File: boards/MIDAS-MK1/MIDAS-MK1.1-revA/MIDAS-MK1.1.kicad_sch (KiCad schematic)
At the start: 105 parts, among them J101 Left, J102 Right, J106 USB4105-GF-A, J107 DM3BT-DSF-PEJS, J108 Conn_01x02, J110 2157601003, J111 2157601003, SW101 SW_Push, SW102 SW_Push, U101 TCAL9539-Q1, U102 TCAL9539-Q1, U103 TCAL9539-Q1, U104 ESP32-S3-WROOM-1U, U105 MCP2518FDT-xSL, U106 MTFCxxxx, U107 TCAN337G, U108 ADS7138-Q1, U109 ECMF02-2AMX6, Y101 40MHz

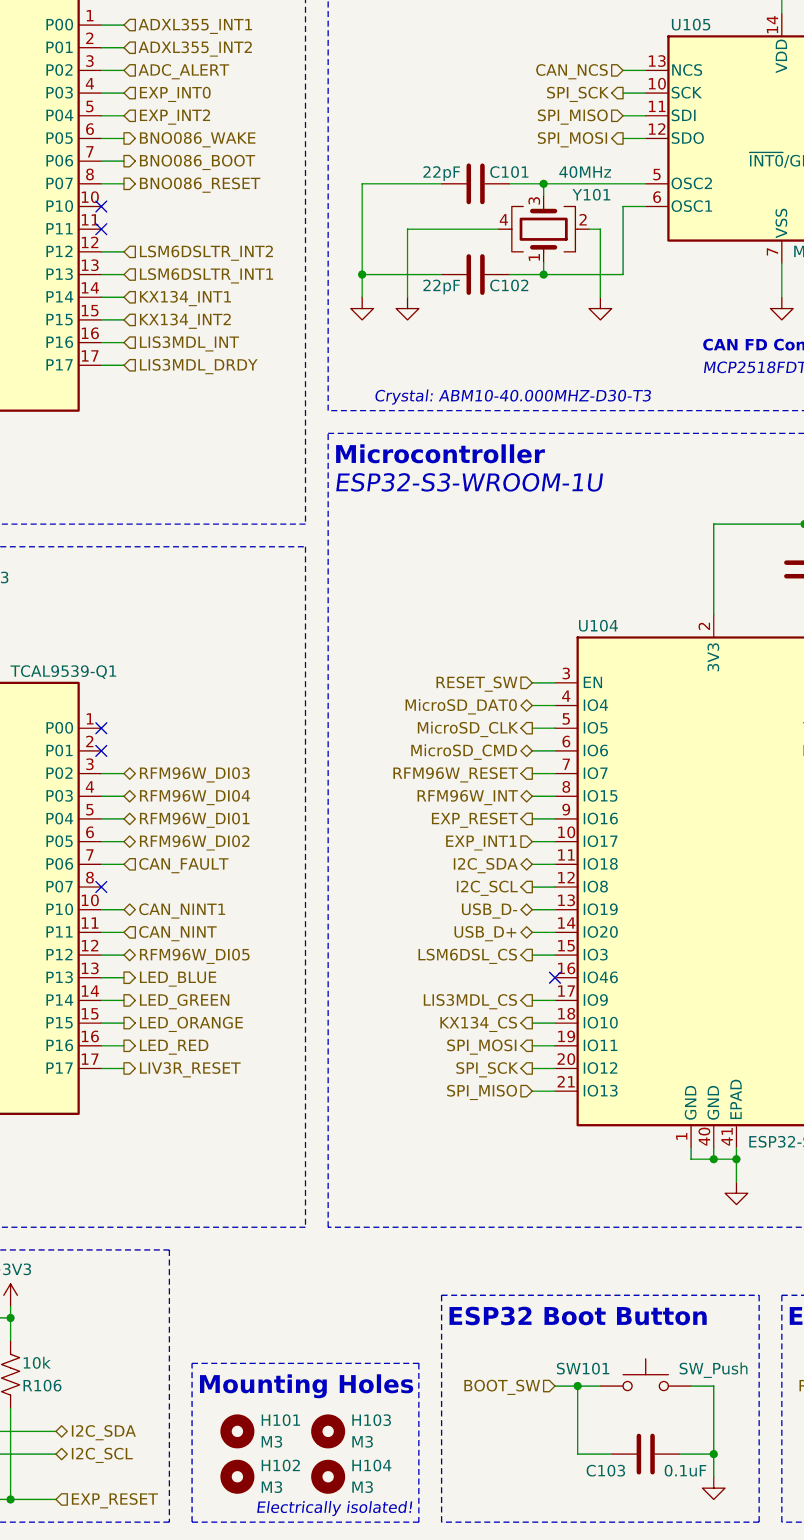
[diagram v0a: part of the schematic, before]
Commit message: Minor Misc formatting/routing changes
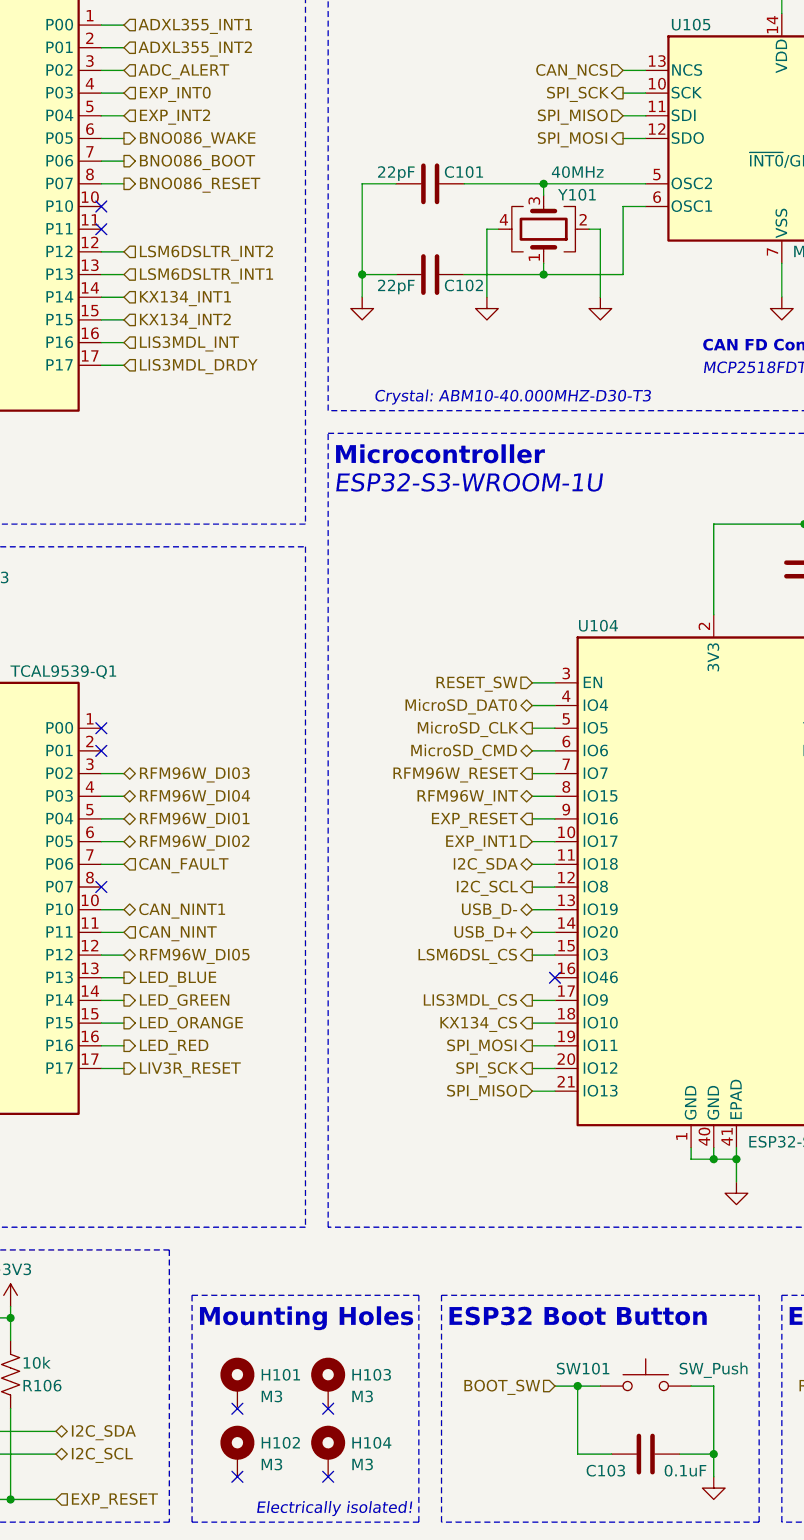
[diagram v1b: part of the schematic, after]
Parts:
- H101, H102, H103, H104: symbol Mechanical:MountingHole -> Mechanical:MountingHole_Pad
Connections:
- no-connect marks 32 -> 36
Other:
- moved on the sheet: C101, C102
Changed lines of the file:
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@@
   (no_connect (at 129.54 58.42))
   (no_connect (at 162.56 53.34))
+  (no_connect (at 76.2 269.24))
   (no_connect (at 304.8 149.86))
   (no_connect (at 162.56 50.8))
@@
   (no_connect (at 129.54 50.8))
   (no_connect (at 129.54 53.34))
+  (no_connect (at 86.36 269.24))
+  (no_connect (at 76.2 276.86))
   (no_connect (at 60.96 134.62))
   (no_connect (at 292.1 154.94))
@@
   (no_connect (at 60.96 137.16))
   (no_connect (at 292.1 152.4))
+  (no_connect (at 86.36 276.86))
   (no_connect (at 162.56 58.42))
   (no_connect (at 162.56 45.72))
@@
     (stroke (width 0) (type default))
   )
-  (wire (pts (xy 110.49 132.08) (xy 106.68 132.08))
+  (wire (pts (xy 110.49 132.08) (xy 101.6 132.08))
     (stroke (width 0) (type default))
   )
@@
     (stroke (width 0) (type default))
   )
-  (wire (pts (xy 110.49 142.24) (xy 106.68 142.24))
+  (wire (pts (xy 110.49 142.24) (xy 101.6 142.24))
     (stroke (width 0) (type default))
   )
@@
     (stroke (width 0) (type default))
   )
-  (wire (pts (xy 99.06 142.24) (xy 90.17 142.24))
+  (wire (pts (xy 93.98 142.24) (xy 90.17 142.24))
     (stroke (width 0) (type default))
   )
@@
     (stroke (width 0) (type default))
   )
-  (wire (pts (xy 99.06 132.08) (xy 90.17 132.08))
+  (wire (pts (xy 93.98 132.08) (xy 90.17 132.08))
     (stroke (width 0) (type default))
   )
@@
     (stroke (width 0) (type default))
   )
-  (wire (pts (xy 105.41 137.16) (xy 95.25 137.16))
+  (wire (pts (xy 104.14 137.16) (xy 105.41 137.16))
     (stroke (width 0) (type default))
   )
@@
     (stroke (width 0) (type default))
   )
-  (wire (pts (xy 95.25 137.16) (xy 95.25 144.78))
+  (wire (pts (xy 104.14 137.16) (xy 104.14 144.78))
     (stroke (width 0) (type default))
   )
@@
     (fill (type none))
   )
-  (rectangle (start 71.12 264.16) (end 96.52 281.94)
+  (rectangle (start 71.12 256.54) (end 96.52 281.94)
     (stroke (width 0) (type dash))
     (fill (type none))
@@
     (effects (font (size 1.27 1.27)) (justify left bottom))
   )
-  (text "Mounting Holes" (at 71.755 267.97 0)
+  (text "Mounting Holes" (at 71.755 260.35 0)
     (effects (font (face "KiCad Font") (size 2 2) (thickness 0.4) bold) (justify left bottom))
   )
@@
     )
   )
-  (symbol (lib_id "Mechanical:MountingHole") (at 86.36 271.78 0) (unit 1)
+  (symbol (lib_id "Mechanical:MountingHole_Pad") (at 86.36 266.7 0) (unit 1)
     (in_bom yes) (on_board yes) (dnp no) (fields_autoplaced)
-    (property "Reference" "H103" (at 88.9 270.5679 0)
+    (property "Reference" "H103" (at 88.9 265.4879 0)
       (effects (font (size 1.27 1.27)) (justify left))
     )
-    (property "Value" "M3" (at 88.9 272.9921 0)
+    (property "Value" "M3" (at 88.9 267.9121 0)
       (effects (font (size 1.27 1.27)) (justify left))
     )
-    (property "Footprint" "MountingHole:MountingHole_3.2mm_M3_Pad_Via" (at 86.36 271.78 0)
+    (property "Footprint" "MountingHole:MountingHole_3.2mm_M3_Pad_Via" (at 86.36 266.7 0)
       (effects (font (size 1.27 1.27)) hide)
     )
-    (property "Datasheet" "~" (at 86.36 271.78 0)
+    (property "Datasheet" "~" (at 86.36 266.7 0)
       (effects (font (size 1.27 1.27)) hide)
     )
+    (pin "1")
     (instances
       (project "MIDAS-MK1.1"
@@
     )
   )
-  (symbol (lib_id "Device:C") (at 102.87 132.08 90) (mirror x) (unit 1)
+  (symbol (lib_id "Device:C") (at 97.79 132.08 90) (mirror x) (unit 1)
     (in_bom yes) (on_board yes) (dnp no)
-    (property "Reference" "C101" (at 106.68 130.81 90)
+    (property "Reference" "C101" (at 101.6 130.81 90)
       (effects (font (size 1.27 1.27)))
     )
-    (property "Value" "22pF" (at 99.06 130.81 90)
+    (property "Value" "22pF" (at 93.98 130.81 90)
       (effects (font (size 1.27 1.27)))
     )
-    (property "Footprint" "Capacitor_SMD:C_0603_1608Metric" (at 106.68 133.0452 0)
+    (property "Footprint" "Capacitor_SMD:C_0603_1608Metric" (at 101.6 133.0452 0)
       (effects (font (size 1.27 1.27)) hide)
     )
-    (property "Datasheet" "~" (at 102.87 132.08 0)
+    (property "Datasheet" "~" (at 97.79 132.08 0)
       (effects (font (size 1.27 1.27)) hide)
     )
@@
     )
   )
-  (symbol (lib_id "power:GND") (at 95.25 144.78 0) (mirror y) (unit 1)
+  (symbol (lib_id "power:GND") (at 104.14 144.78 0) (mirror y) (unit 1)
     (in_bom yes) (on_board yes) (dnp no) (fields_autoplaced)
-    (property "Reference" "#PWR0113" (at 95.25 151.13 0)
+    (property "Reference" "#PWR0113" (at 104.14 151.13 0)
       (effects (font (size 1.27 1.27)) hide)
     )
-    (property "Value" "GND" (at 95.25 148.9131 0)
+    (property "Value" "GND" (at 104.14 148.9131 0)
       (effects (font (size 1.27 1.27)) hide)
     )
-    (property "Footprint" "" (at 95.25 144.78 0)
+    (property "Footprint" "" (at 104.14 144.78 0)
       (effects (font (size 1.27 1.27)) hide)
     )
-    (property "Datasheet" "" (at 95.25 144.78 0)
+    (property "Datasheet" "" (at 104.14 144.78 0)
       (effects (font (size 1.27 1.27)) hide)
     )
@@
     )
   )
-  (symbol (lib_id "Device:C") (at 102.87 142.24 270) (mirror x) (unit 1)
+  (symbol (lib_id "Device:C") (at 97.79 142.24 270) (mirror x) (unit 1)
     (in_bom yes) (on_board yes) (dnp no)
-    (property "Reference" "C102" (at 106.68 143.51 90)
+    (property "Reference" "C102" (at 101.6 143.51 90)
       (effects (font (size 1.27 1.27)))
     )
-    (property "Value" "22pF" (at 99.06 143.51 90)
+    (property "Value" "22pF" (at 93.98 143.51 90)
       (effects (font (size 1.27 1.27)))
     )
-    (property "Footprint" "Capacitor_SMD:C_0603_1608Metric" (at 99.06 141.2748 0)
+    (property "Footprint" "Capacitor_SMD:C_0603_1608Metric" (at 93.98 141.2748 0)
       (effects (font (size 1.27 1.27)) hide)
     )
-    (property "Datasheet" "~" (at 102.87 142.24 0)
+    (property "Datasheet" "~" (at 97.79 142.24 0)
       (effects (font (size 1.27 1.27)) hide)
     )
@@
     )
   )
-  (symbol (lib_id "Mechanical:MountingHole") (at 86.36 276.86 0) (unit 1)
+  (symbol (lib_id "Mechanical:MountingHole_Pad") (at 86.36 274.32 0) (unit 1)
     (in_bom yes) (on_board yes) (dnp no) (fields_autoplaced)
-    (property "Reference" "H104" (at 88.9 275.6479 0)
+    (property "Reference" "H104" (at 88.9 273.1079 0)
       (effects (font (size 1.27 1.27)) (justify left))
     )
-    (property "Value" "M3" (at 88.9 278.0721 0)
+    (property "Value" "M3" (at 88.9 275.5321 0)
       (effects (font (size 1.27 1.27)) (justify left))
     )
-    (property "Footprint" "MountingHole:MountingHole_3.2mm_M3_Pad_Via" (at 86.36 276.86 0)
+    (property "Footprint" "MountingHole:MountingHole_3.2mm_M3_Pad_Via" (at 86.36 274.32 0)
       (effects (font (size 1.27 1.27)) hide)
     )
-    (property "Datasheet" "~" (at 86.36 276.86 0)
+    (property "Datasheet" "~" (at 86.36 274.32 0)
       (effects (font (size 1.27 1.27)) hide)
     )
+    (pin "1")
     (instances
       (project "MIDAS-MK1.1"
@@
     )
   )
-  (symbol (lib_id "Mechanical:MountingHole") (at 76.2 271.78 0) (unit 1)
+  (symbol (lib_id "Mechanical:MountingHole_Pad") (at 76.2 266.7 0) (unit 1)
     (in_bom yes) (on_board yes) (dnp no) (fields_autoplaced)
-    (property "Reference" "H101" (at 78.74 270.5679 0)
+    (property "Reference" "H101" (at 78.74 265.4879 0)
       (effects (font (size 1.27 1.27)) (justify left))
     )
-    (property "Value" "M3" (at 78.74 272.9921 0)
+    (property "Value" "M3" (at 78.74 267.9121 0)
       (effects (font (size 1.27 1.27)) (justify left))
     )
-    (property "Footprint" "MountingHole:MountingHole_3.2mm_M3_Pad_Via" (at 76.2 271.78 0)
+    (property "Footprint" "MountingHole:MountingHole_3.2mm_M3_Pad_Via" (at 76.2 266.7 0)
       (effects (font (size 1.27 1.27)) hide)
     )
-    (property "Datasheet" "~" (at 76.2 271.78 0)
+    (property "Datasheet" "~" (at 76.2 266.7 0)
       (effects (font (size 1.27 1.27)) hide)
     )
+    (pin "1")
     (instances
       (project "MIDAS-MK1.1"
@@
   (symbol (lib_id "Device:Crystal_GND24") (at 110.49 137.16 270) (mirror x) (unit 1)
     (in_bom yes) (on_board yes) (dnp no)
-    (property "Reference" "Y101" (at 118.11 133.35 90)
-      (effects (font (size 1.27 1.27)) (justify right))
+    (property "Reference" "Y101" (at 114.3 133.35 90)
+      (effects (font (size 1.27 1.27)))
     )
-    (property "Value" "40MHz" (at 118.11 130.81 90)
-      (effects (font (size 1.27 1.27)) (justify right))
+    (property "Value" "40MHz" (at 114.3 130.81 90)
+      (effects (font (size 1.27 1.27)))
     )
     (property "Footprint" "Crystal:Crystal_SMD_Abracon_ABM10-4Pin_2.5x2.0mm" (at 110.49 137.16 0)
@@
     )
   )
-  (symbol (lib_id "Mechanical:MountingHole") (at 76.2 276.86 0) (unit 1)
+  (symbol (lib_id "Mechanical:MountingHole_Pad") (at 76.2 274.32 0) (unit 1)
     (in_bom yes) (on_board yes) (dnp no) (fields_autoplaced)
-    (property "Reference" "H102" (at 78.74 275.6479 0)
+    (property "Reference" "H102" (at 78.74 273.1079 0)
       (effects (font (size 1.27 1.27)) (justify left))
     )
-    (property "Value" "M3" (at 78.74 278.0721 0)
+    (property "Value" "M3" (at 78.74 275.5321 0)
       (effects (font (size 1.27 1.27)) (justify left))
     )
-    (property "Footprint" "MountingHole:MountingHole_3.2mm_M3_Pad_Via" (at 76.2 276.86 0)
+    (property "Footprint" "MountingHole:MountingHole_3.2mm_M3_Pad_Via" (at 76.2 274.32 0)
       (effects (font (size 1.27 1.27)) hide)
     )
-    (property "Datasheet" "~" (at 76.2 276.86 0)
+    (property "Datasheet" "~" (at 76.2 274.32 0)
       (effects (font (size 1.27 1.27)) hide)
     )
+    (pin "1")
     (instances
       (project "MIDAS-MK1.1"
